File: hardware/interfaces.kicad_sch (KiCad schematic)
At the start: 2 parts, among them J3 SSQ-126-04-G-D, J4 SSQ-126-04-G-D

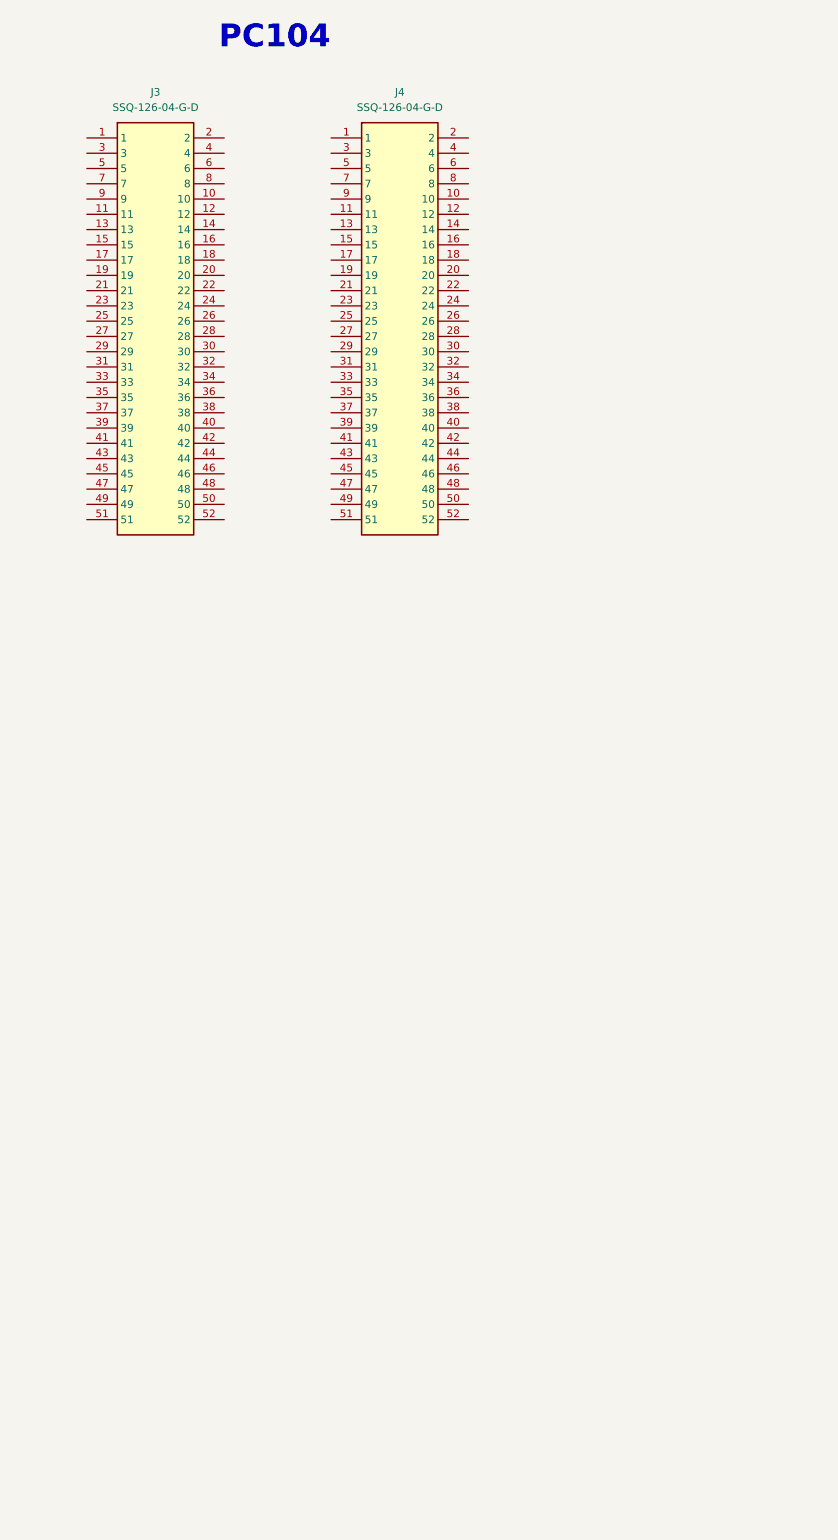
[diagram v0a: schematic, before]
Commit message: updated hardware
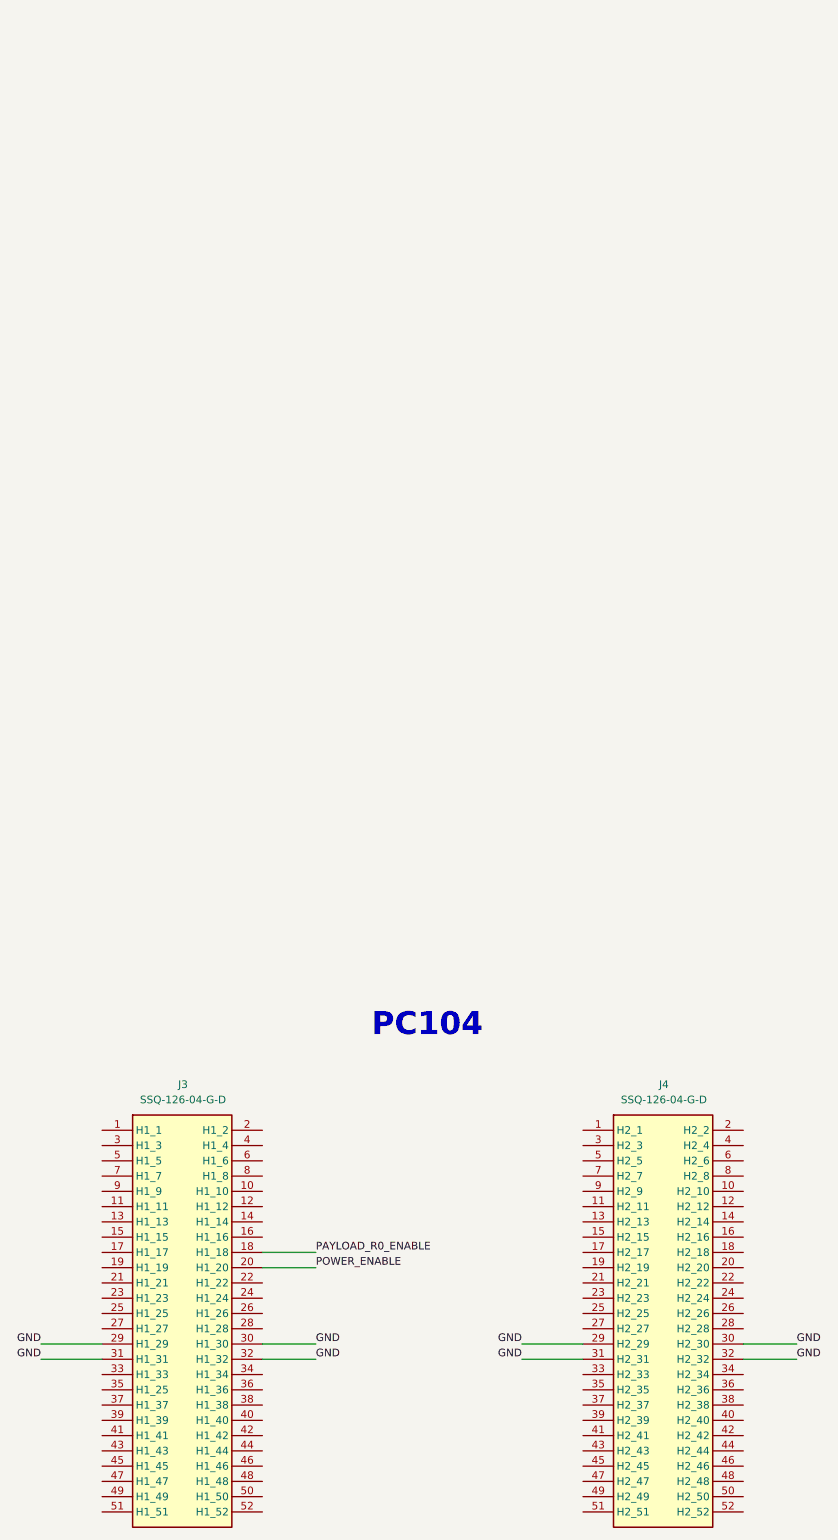
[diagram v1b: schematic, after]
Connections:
- net PAYLOAD_R0_ENABLE: now reaches J3.18 (H1_18)
- net POWER_ENABLE: now reaches J3.20 (H1_20)
- net GND: now reaches J3.29 (H1_29)
- net GND: now also J3.30 (H1_30), J3.31 (H1_31), J3.32 (H1_32), J4.29 (H2_29), J4.30 (H2_30), J4.31 (H2_31), J4.32 (H2_32)
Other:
- moved on the sheet: J3
